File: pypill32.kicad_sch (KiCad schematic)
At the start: 43 parts, among them J1 HeaderR, J2 HeaderL, J4 ISP, SW1 RST_BTN, SW2 BOOT_BTN, U1 SRV05-4, U2 PY32F030F18P6, U3 CH340N, U4 AMS1117-3.3, Y1 32.768 kHz

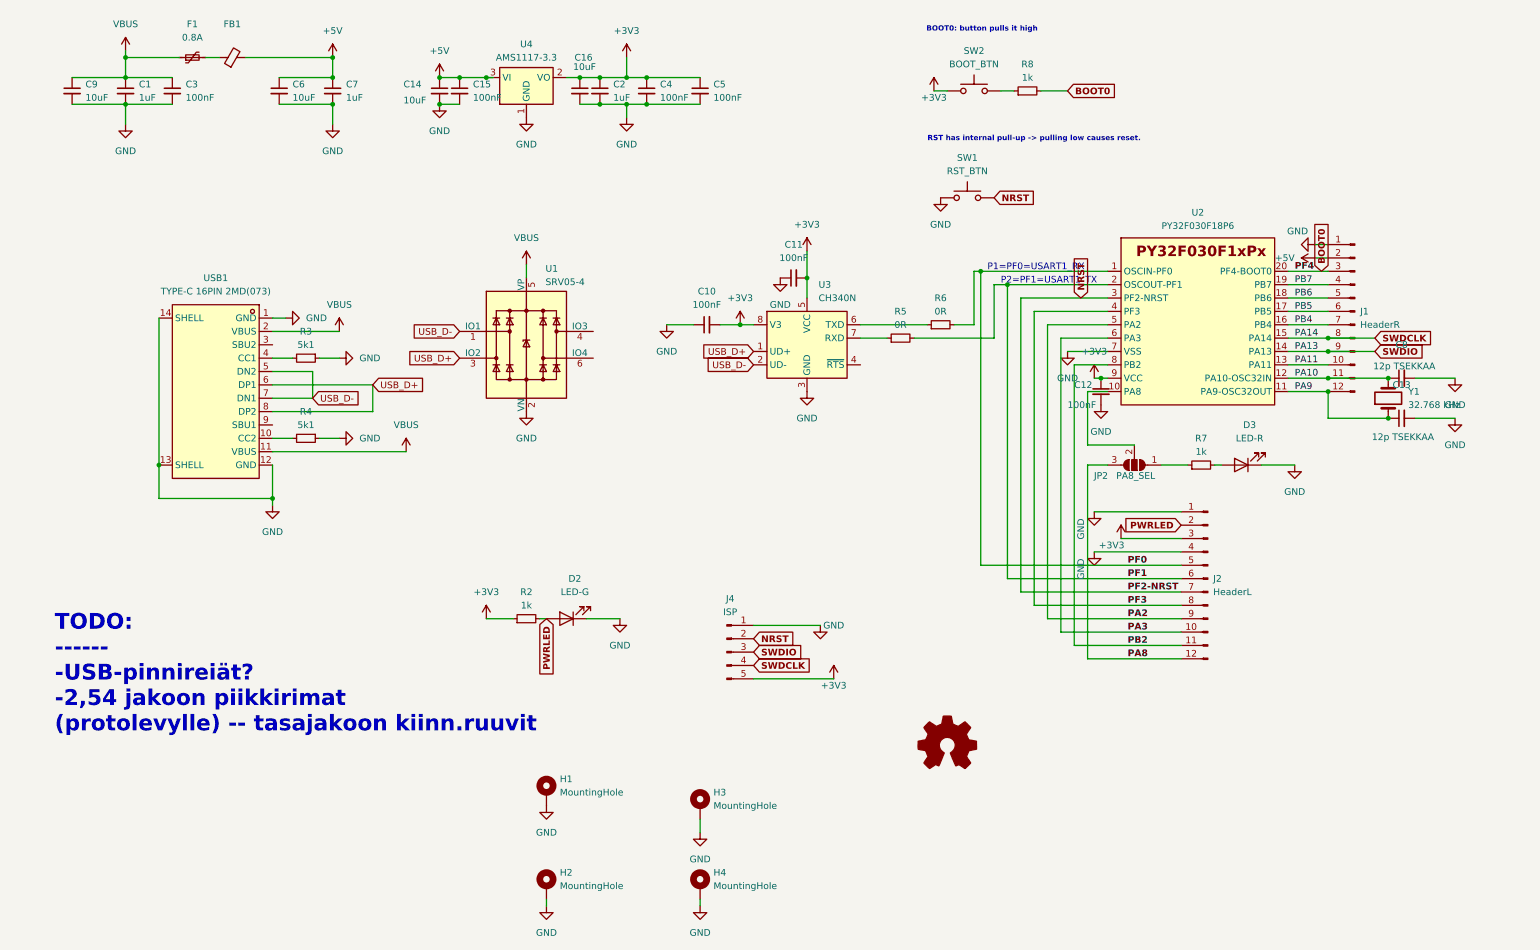
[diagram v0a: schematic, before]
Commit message: checking and verifying still
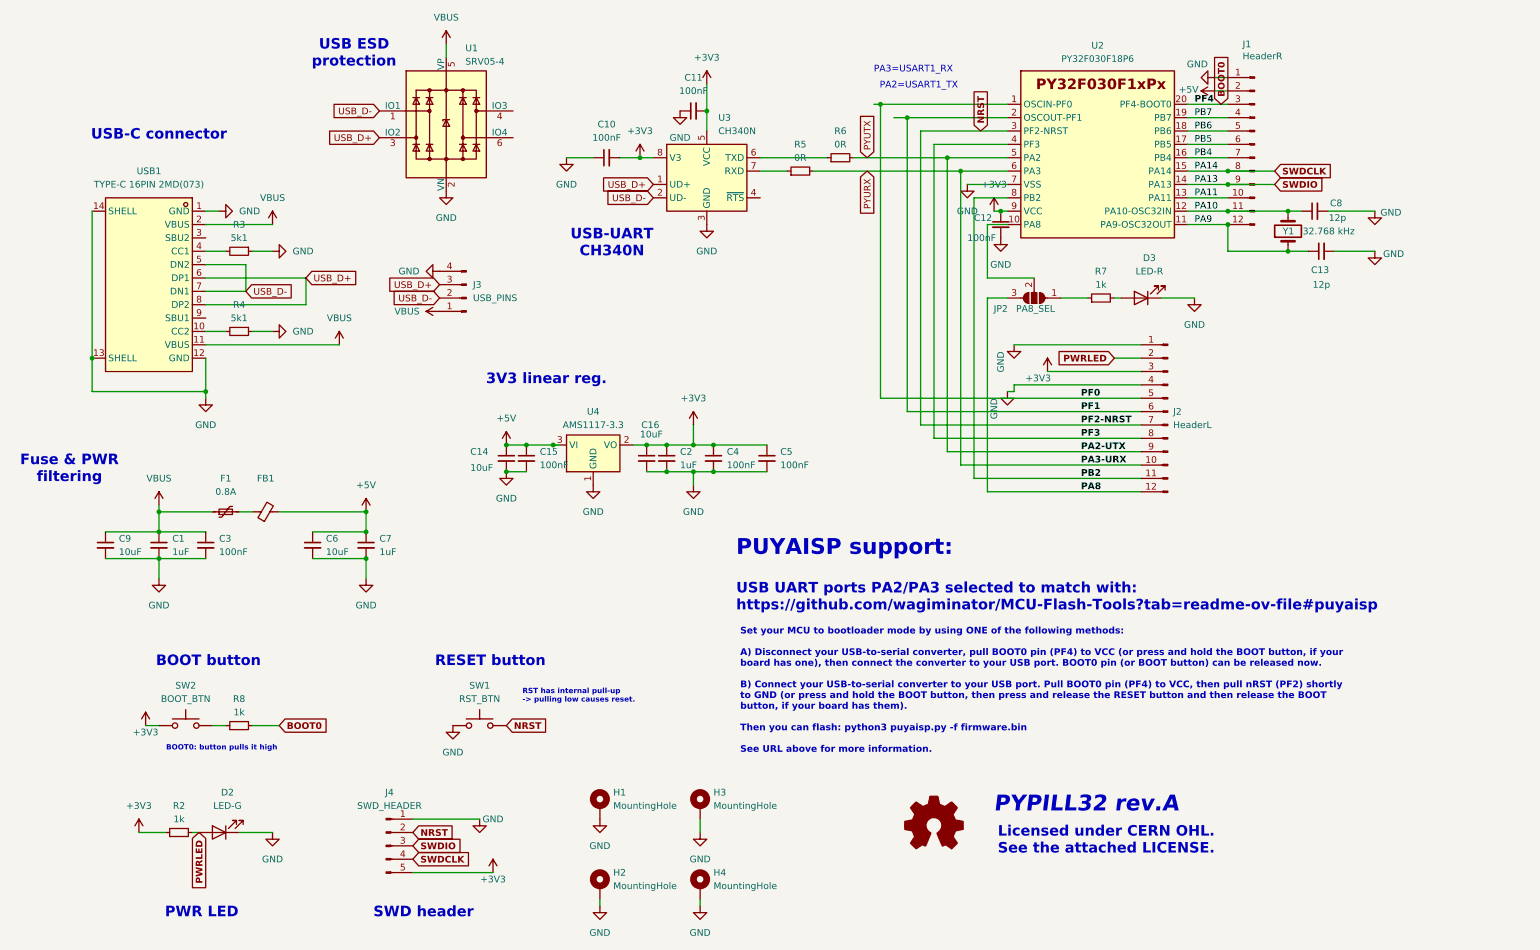
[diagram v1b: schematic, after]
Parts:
- added J3: USB_PINS, Connector_PinHeader_2.00mm:PinHeader_1x04_P2.00mm_Vertical, symbol Connector:Conn_01x04_Pin
- C13, C8: value 12p TSEKKAA -> 12p
- J4: value ISP -> SWD_HEADER
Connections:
- net GND: now also J3.4 (Pin_4)
- net PF0: no longer R6.2
- net PF1: no longer R5.2
- net USB_D+: now also J3.3 (Pin_3)
- net USB_D-: now also J3.2 (Pin_2)
- net VBUS: now also J3.1 (Pin_1)
- net PA2 renamed PYUTX
- net PYUTX: now also R6.2
- net PA3 renamed PYURX
- net PYURX: now also R5.2
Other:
- note added: "3V3 linear reg."
- note added: "BOOT button"
- note added: "Fuse & PWR filtering"
- note added: "Licensed under CERN OHL. See the attached LICENSE."
- note added: "PA2=USART1_TX"
- note added: "PA3=USART1_RX"
- note added: "PUYAISP support:"
- note added: "PWR LED"
- note added: "PYPILL32 rev.A"
- note added: "RESET button"
- note added: "SWD header"
- note added: "Set your MCU to bootloader mode by using ONE of the following methods: A) Disconnect your USB-to-serial converter, pull BOOT0 pin (PF4) to VCC (or press and hold the BOOT button, if your board has one), then connect the converter to your USB port. BOOT0 pin (or BOOT button) can be released now. B) Connect your USB-to-serial converter to your USB port. Pull BOOT0 pin (PF4) to VCC, then pull nRST (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"
- note added: "USB ESD protection"
- note added: "USB UART ports PA2/PA3 selected to match with: https://github.com/wagiminator/MCU-Flash-Tools?tab=readme-ov-file#puyaisp"
- note added: "USB-C connector"
- note added: "USB-UART CH340N"
- note removed: "P1=PF0=USART1_RX"
- note removed: "P2=PF1=USART1_TX"
- note removed: "TODO: ------ -USB-pinnireiät? -2,54 jakoon piikkirimat (protolevylle) -- tasajakoon kiinn.ruuvit"
- title: (none) -> pypill32 - indie py32f030 evaluation board
- moved on the sheet: C1, C10, C11, C12, C13, C14, C15, C16, C2, C3, C4, C5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
